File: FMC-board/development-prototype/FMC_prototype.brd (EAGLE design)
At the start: 103.8 x 69.8 mm, 65 parts, among them J1 DC_POWER_JACK-PJ-102AH, J2 DC_POWER_JACK-PJ-102AH

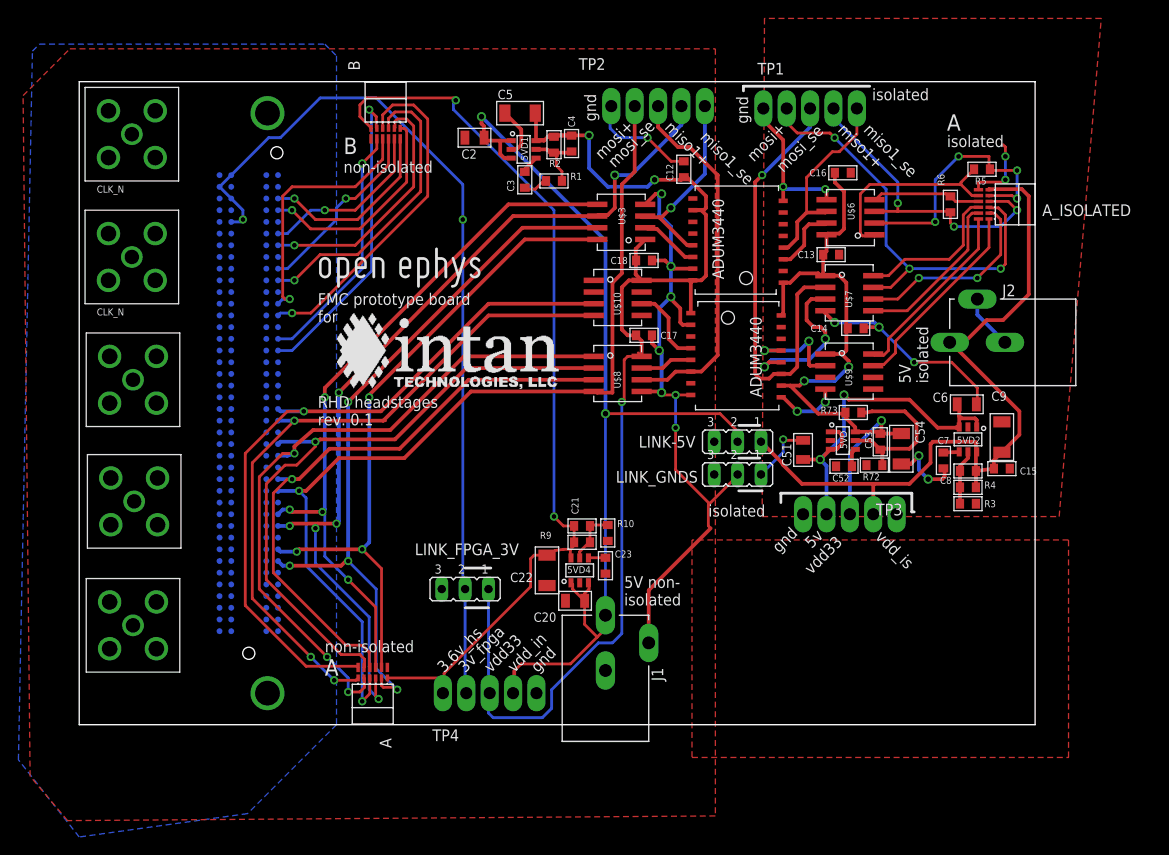
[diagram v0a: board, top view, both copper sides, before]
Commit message: small cleanups
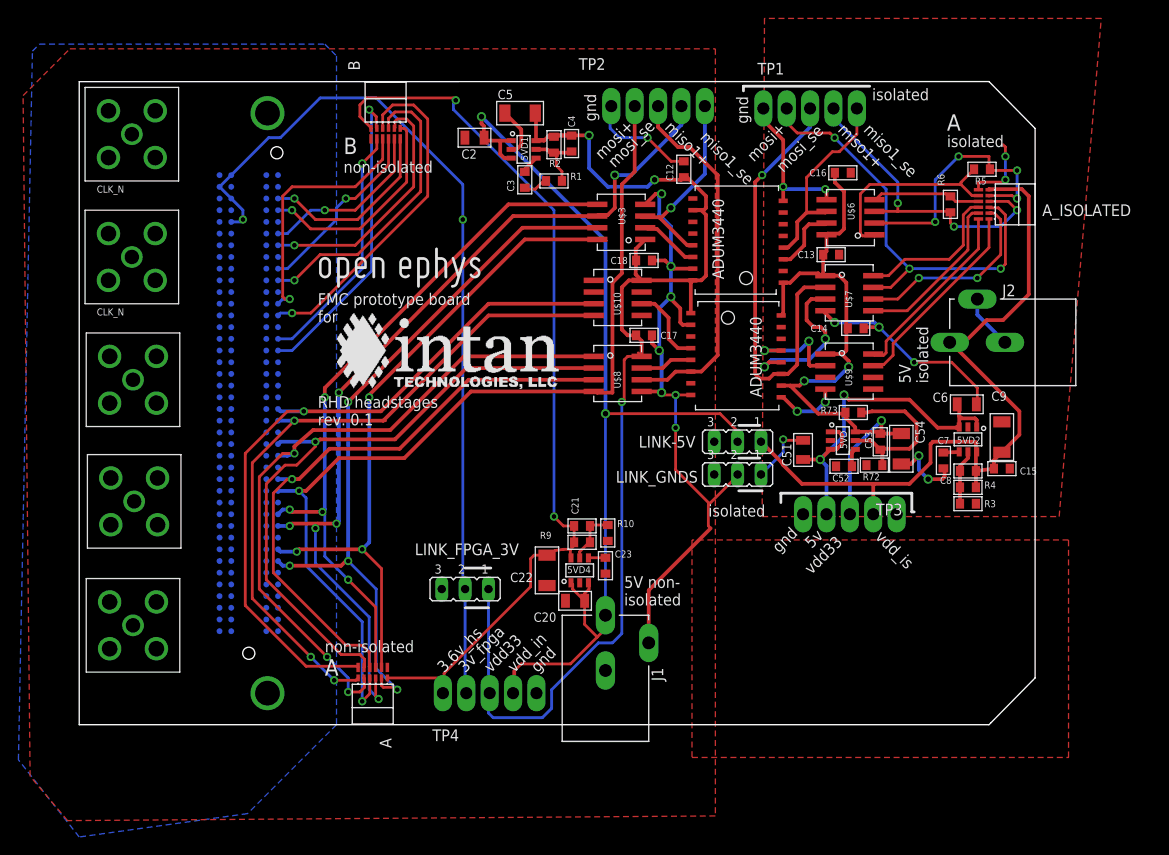
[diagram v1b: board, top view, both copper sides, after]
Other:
- outline, holes or cut-outs redrawn
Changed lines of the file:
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@@
 <setting verticaltext="up"/>
 </settings>
-<grid distance="0.01" unitdist="inch" unit="inch" style="dots" multiple="1" display="yes" altdistance="0.0125" altunitdist="inch" altunit="inch"/>
+<grid distance="0.01" unitdist="inch" unit="inch" style="lines" multiple="1" display="yes" altdistance="0.0125" altunitdist="inch" altunit="inch"/>
 <layers>
 <layer number="1" name="Top" color="42" fill="1" visible="yes" active="yes"/>
@@
 <board>
 <plain>
-<wire x1="0" y1="0" x2="103.81" y2="0" width="0" layer="20"/>
-<wire x1="103.81" y1="0" x2="103.81" y2="69.84" width="0" layer="20"/>
-<wire x1="103.81" y1="69.84" x2="0" y2="69.84" width="0" layer="20"/>
+<wire x1="0" y1="0" x2="98.806" y2="0" width="0" layer="20"/>
+<wire x1="98.806" y1="0" x2="98.984" y2="0.178" width="0" layer="20"/>
+<wire x1="98.984" y1="0.178" x2="103.81" y2="5.08" width="0" layer="20"/>
+<wire x1="103.81" y1="5.08" x2="103.81" y2="64.76" width="0" layer="20"/>
+<wire x1="103.81" y1="64.76" x2="98.816" y2="69.84" width="0" layer="20"/>
+<wire x1="98.816" y1="69.84" x2="98.806" y2="69.85" width="0" layer="20"/>
+<wire x1="98.806" y1="69.85" x2="0" y2="69.84" width="0" layer="20"/>
 <wire x1="0" y1="69.84" x2="0" y2="0" width="0" layer="20"/>
 <text x="1.905" y="57.785" size="0.762" layer="21">CLK_N</text>
@@
 <wire x1="57.658" y1="64.77" x2="57.658" y2="67.056" width="0.3048" layer="16"/>
 <wire x1="57.658" y1="67.056" x2="57.785" y2="67.183" width="0.3048" layer="16"/>
+<wire x1="21.59" y1="50.8" x2="21.59" y2="54.61" width="0" layer="19" extent="16-16"/>
+<wire x1="21.59" y1="46.99" x2="21.59" y2="50.8" width="0" layer="19" extent="16-16"/>
+<wire x1="21.59" y1="39.37" x2="21.59" y2="43.18" width="0" layer="19" extent="16-16"/>
 <wire x1="21.59" y1="27.94" x2="21.59" y2="31.75" width="0" layer="19" extent="16-16"/>
 <wire x1="21.59" y1="24.13" x2="21.59" y2="27.94" width="0" layer="19" extent="16-16"/>
+<wire x1="15.24" y1="54.61" x2="21.59" y2="54.61" width="0" layer="19" extent="16-16"/>
 </signal>
 <signal name="MISO2+">
@@
 <contactref element="A_ISOLATED" pad="T1"/>
 <wire x1="97.663" y1="54.9275" x2="97.663" y2="51.689" width="0.3048" layer="1"/>
-<wire x1="97.663" y1="51.689" x2="87.884" y2="41.91" width="0.3048" layer="1"/>
-<wire x1="87.884" y1="41.91" x2="87.884" y2="40.64" width="0.3048" layer="1"/>
-<wire x1="87.884" y1="40.64" x2="87.376" y2="40.132" width="0.3048" layer="1"/>
+<wire x1="97.663" y1="51.689" x2="87.63" y2="41.656" width="0.3048" layer="1"/>
+<wire x1="87.63" y1="41.656" x2="87.63" y2="40.386" width="0.3048" layer="1"/>
+<wire x1="87.63" y1="40.386" x2="87.376" y2="40.132" width="0.3048" layer="1"/>
 <wire x1="87.376" y1="40.132" x2="86.353" y2="40.132" width="0.3048" layer="1"/>
 <wire x1="86.353" y1="40.132" x2="86.226" y2="40.259" width="0.3048" layer="1"/>
@@
 <wire x1="81.026" y1="47.498" x2="78.74" y2="47.498" width="0.4064" layer="1"/>
 <wire x1="78.74" y1="47.498" x2="77.978" y2="46.736" width="0.4064" layer="1"/>
-<wire x1="77.978" y1="46.736" x2="77.978" y2="38.862" width="0.4064" layer="1"/>
-<wire x1="77.978" y1="38.862" x2="77.216" y2="38.1" width="0.4064" layer="1"/>
-<wire x1="77.216" y1="38.1" x2="76.235" y2="38.1" width="0.4064" layer="1"/>
+<wire x1="77.978" y1="46.736" x2="77.978" y2="39.116" width="0.4064" layer="1"/>
+<wire x1="77.978" y1="39.116" x2="76.962" y2="38.1" width="0.4064" layer="1"/>
+<wire x1="76.962" y1="38.1" x2="76.235" y2="38.1" width="0.4064" layer="1"/>
 <wire x1="79.375" y1="66.929" x2="79.375" y2="64.897" width="0.4064" layer="16"/>
 <wire x1="79.375" y1="64.897" x2="74.168" y2="59.69" width="0.4064" layer="16"/>
@@
 <contactref element="U$9" pad="P7"/>
 <wire x1="98.806" y1="54.9275" x2="98.806" y2="51.816" width="0.3048" layer="1"/>
-<wire x1="98.806" y1="51.816" x2="88.646" y2="41.656" width="0.3048" layer="1"/>
-<wire x1="88.646" y1="41.656" x2="88.646" y2="40.386" width="0.3048" layer="1"/>
-<wire x1="88.646" y1="40.386" x2="87.376" y2="39.116" width="0.3048" layer="1"/>
+<wire x1="98.806" y1="51.816" x2="88.392" y2="41.402" width="0.3048" layer="1"/>
+<wire x1="88.392" y1="41.402" x2="88.392" y2="40.132" width="0.3048" layer="1"/>
+<wire x1="88.392" y1="40.132" x2="87.376" y2="39.116" width="0.3048" layer="1"/>
 <wire x1="87.376" y1="39.116" x2="86.353" y2="39.116" width="0.3048" layer="1"/>
 <wire x1="86.353" y1="39.116" x2="86.226" y2="38.989" width="0.3048" layer="1"/>

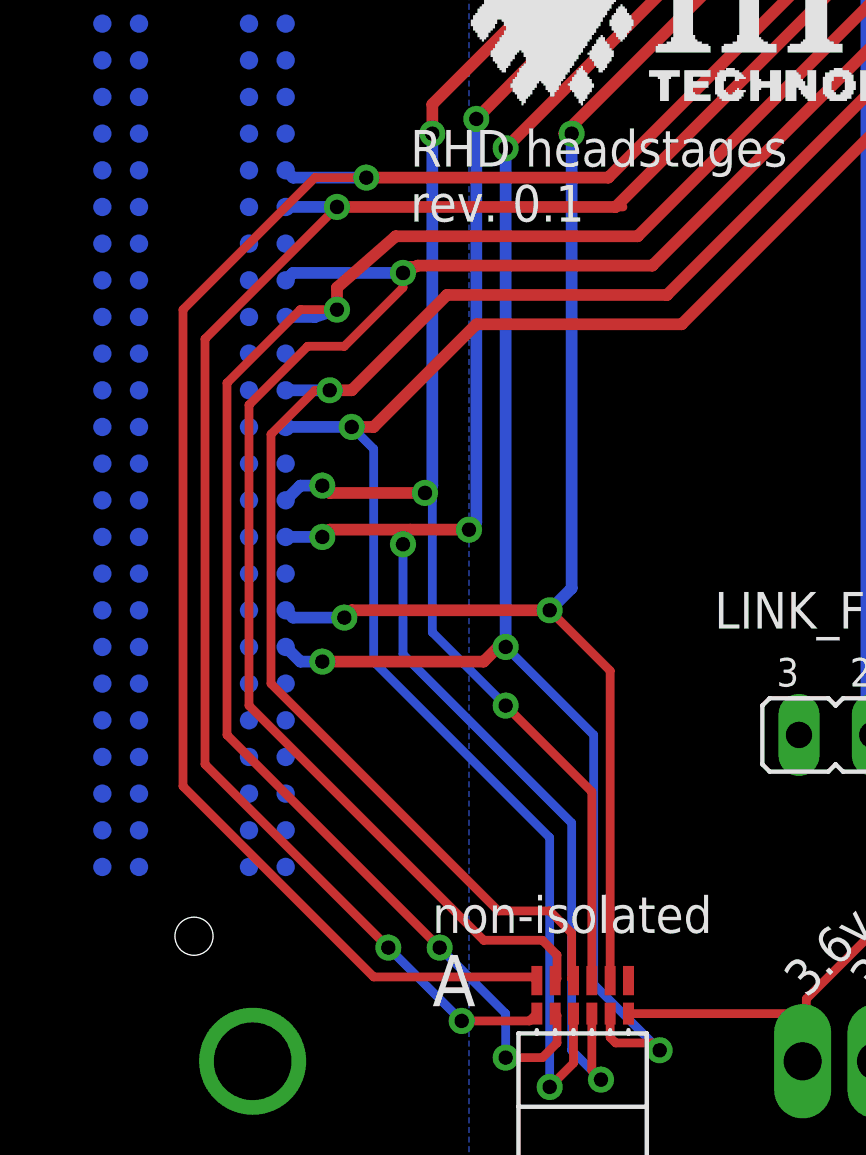
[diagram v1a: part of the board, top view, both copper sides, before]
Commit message: more small cleanups
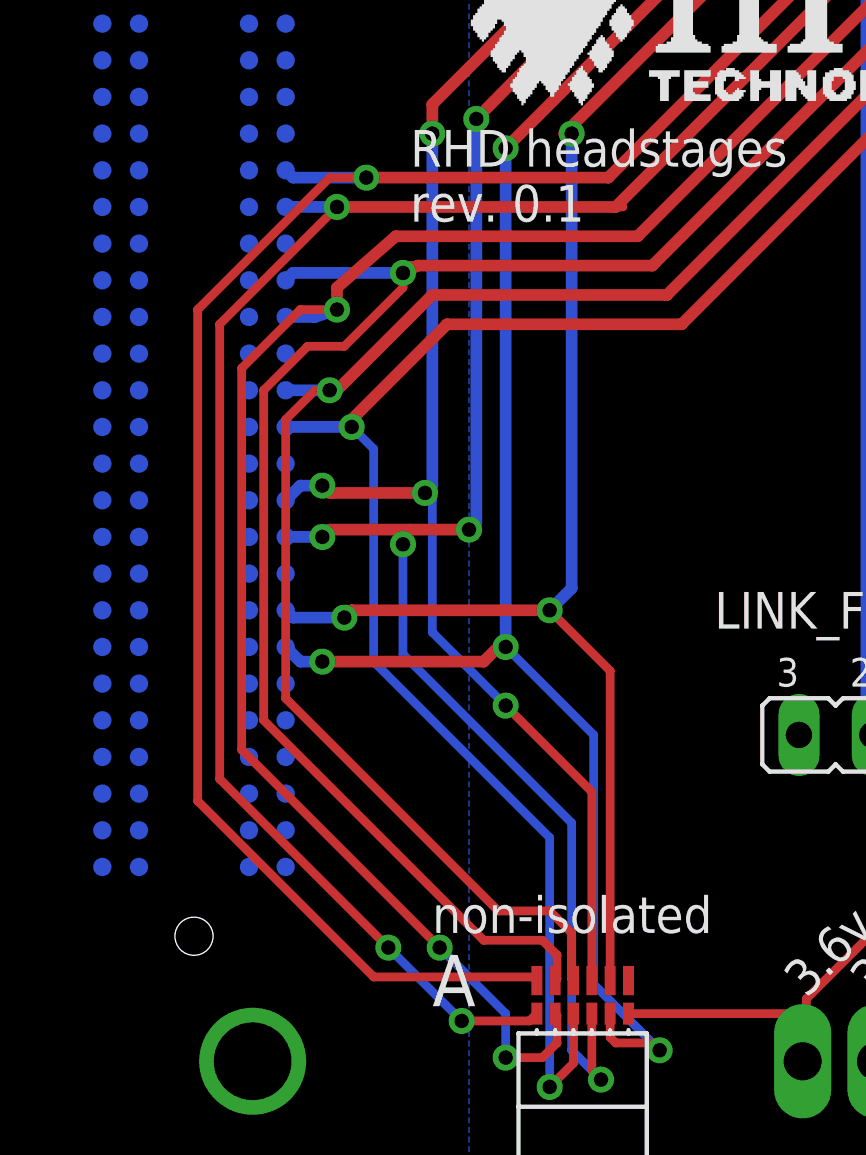
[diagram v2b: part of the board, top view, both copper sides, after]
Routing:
- net MOSI-: track 66.5 -> 65.6 mm
- net CS-: track 79.0 -> 78.3 mm
- net MOSI+: track 101.5 -> 102.0 mm
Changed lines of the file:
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@@
 <setting verticaltext="up"/>
 </settings>
-<grid distance="0.01" unitdist="inch" unit="inch" style="lines" multiple="1" display="yes" altdistance="0.0125" altunitdist="inch" altunit="inch"/>
+<grid distance="0.02" unitdist="inch" unit="inch" style="lines" multiple="1" display="yes" altdistance="0.0125" altunitdist="inch" altunit="inch"/>
 <layers>
 <layer number="1" name="Top" color="42" fill="1" visible="yes" active="yes"/>
-<layer number="16" name="Bottom" color="1" fill="1" visible="yes" active="yes"/>
+<layer number="16" name="Bottom" color="1" fill="1" visible="no" active="yes"/>
 <layer number="17" name="Pads" color="2" fill="1" visible="yes" active="yes"/>
 <layer number="18" name="Vias" color="2" fill="1" visible="yes" active="yes"/>
@@
 <wire x1="25.654" y1="30.226" x2="23.622" y2="28.194" width="0.3048" layer="1"/>
 <wire x1="23.622" y1="28.194" x2="22.352" y2="28.194" width="0.3048" layer="1"/>
-<wire x1="22.352" y1="28.194" x2="20.32" y2="26.162" width="0.3048" layer="1"/>
-<wire x1="20.32" y1="26.162" x2="20.32" y2="15.748" width="0.3048" layer="1"/>
-<wire x1="20.32" y1="15.748" x2="28.448" y2="7.62" width="0.3048" layer="1"/>
+<wire x1="22.352" y1="28.194" x2="20.828" y2="26.67" width="0.3048" layer="1"/>
+<wire x1="20.828" y1="26.67" x2="20.828" y2="15.24" width="0.3048" layer="1"/>
+<wire x1="20.828" y1="15.24" x2="28.448" y2="7.62" width="0.3048" layer="1"/>
 <wire x1="28.448" y1="7.62" x2="30.48" y2="7.62" width="0.3048" layer="1"/>
 <wire x1="30.48" y1="7.62" x2="30.988" y2="7.112" width="0.3048" layer="1"/>
@@
 <wire x1="22.606" y1="29.21" x2="21.59" y2="29.21" width="0.4064" layer="16"/>
 <wire x1="23.368" y1="29.464" x2="22.098" y2="29.464" width="0.3048" layer="1"/>
-<wire x1="22.098" y1="29.464" x2="19.558" y2="26.924" width="0.3048" layer="1"/>
-<wire x1="19.558" y1="26.924" x2="19.558" y2="14.732" width="0.3048" layer="1"/>
-<wire x1="19.558" y1="14.732" x2="26.924" y2="7.366" width="0.3048" layer="1"/>
+<wire x1="22.098" y1="29.464" x2="20.066" y2="27.432" width="0.3048" layer="1"/>
+<wire x1="20.066" y1="27.432" x2="20.066" y2="14.224" width="0.3048" layer="1"/>
+<wire x1="20.066" y1="14.224" x2="26.924" y2="7.366" width="0.3048" layer="1"/>
 <via x="26.924" y="7.366" extent="1-16" drill="0.5"/>
 <wire x1="26.924" y1="7.366" x2="29.21" y2="5.08" width="0.3048" layer="16"/>
@@
 <wire x1="55.88" y1="37.465" x2="42.291" y2="37.465" width="0.4064" layer="1"/>
 <wire x1="42.291" y1="37.465" x2="34.798" y2="29.972" width="0.4064" layer="1"/>
-<wire x1="34.798" y1="29.972" x2="27.178" y2="29.972" width="0.4064" layer="1"/>
-<wire x1="27.178" y1="29.972" x2="23.876" y2="26.67" width="0.4064" layer="1"/>
-<wire x1="23.876" y1="26.67" x2="23.114" y2="26.67" width="0.4064" layer="1"/>
+<wire x1="34.798" y1="29.972" x2="26.67" y2="29.972" width="0.4064" layer="1"/>
+<wire x1="26.67" y1="29.972" x2="23.368" y2="26.67" width="0.4064" layer="1"/>
+<wire x1="23.368" y1="26.67" x2="23.114" y2="26.67" width="0.4064" layer="1"/>
 <via x="23.114" y="26.67" extent="1-16" drill="0.5"/>
 <wire x1="23.114" y1="26.67" x2="21.59" y2="26.67" width="0.4064" layer="16"/>
-<wire x1="23.876" y1="26.67" x2="22.606" y2="26.67" width="0.3048" layer="1"/>
-<wire x1="22.606" y1="26.67" x2="21.082" y2="25.146" width="0.3048" layer="1"/>
-<wire x1="21.082" y1="25.146" x2="21.082" y2="16.51" width="0.3048" layer="1"/>
-<wire x1="21.082" y1="16.51" x2="28.956" y2="8.636" width="0.3048" layer="1"/>
+<wire x1="23.368" y1="26.67" x2="22.606" y2="26.67" width="0.3048" layer="1"/>
+<wire x1="22.606" y1="26.67" x2="21.59" y2="25.654" width="0.3048" layer="1"/>
+<wire x1="21.59" y1="25.654" x2="21.59" y2="16.002" width="0.3048" layer="1"/>
+<wire x1="21.59" y1="16.002" x2="28.956" y2="8.636" width="0.3048" layer="1"/>
 <wire x1="28.956" y1="8.636" x2="30.734" y2="8.636" width="0.3048" layer="1"/>
 <wire x1="30.734" y1="8.636" x2="31.496" y2="7.874" width="0.3048" layer="1"/>
@@
 <wire x1="55.88" y1="36.195" x2="42.545" y2="36.195" width="0.4064" layer="1"/>
 <wire x1="42.545" y1="36.195" x2="35.306" y2="28.956" width="0.4064" layer="1"/>
-<wire x1="35.306" y1="28.956" x2="28.194" y2="28.956" width="0.4064" layer="1"/>
-<wire x1="28.194" y1="28.956" x2="24.638" y2="25.4" width="0.4064" layer="1"/>
-<wire x1="24.638" y1="25.4" x2="23.876" y2="25.4" width="0.4064" layer="1"/>
+<wire x1="35.306" y1="28.956" x2="27.178" y2="28.956" width="0.4064" layer="1"/>
+<wire x1="27.178" y1="28.956" x2="23.622" y2="25.4" width="0.4064" layer="1"/>
+<wire x1="23.622" y1="25.4" x2="23.876" y2="25.4" width="0.4064" layer="1"/>
 <via x="23.876" y="25.4" extent="1-16" drill="0.5"/>
 <wire x1="23.876" y1="25.4" x2="21.59" y2="25.4" width="0.4064" layer="16"/>
@@
 <wire x1="24.384" y1="34.036" x2="21.844" y2="34.036" width="0.4064" layer="16"/>
 <wire x1="21.844" y1="34.036" x2="21.59" y2="34.29" width="0.4064" layer="16"/>
-<wire x1="24.384" y1="34.036" x2="22.606" y2="34.036" width="0.3048" layer="1"/>
-<wire x1="22.606" y1="34.036" x2="18.034" y2="29.464" width="0.3048" layer="1"/>
-<wire x1="18.034" y1="29.464" x2="18.034" y2="12.954" width="0.3048" layer="1"/>
-<wire x1="18.034" y1="12.954" x2="24.638" y2="6.35" width="0.3048" layer="1"/>
+<wire x1="24.384" y1="34.036" x2="23.114" y2="34.036" width="0.3048" layer="1"/>
+<wire x1="23.114" y1="34.036" x2="18.542" y2="29.464" width="0.3048" layer="1"/>
+<wire x1="18.542" y1="29.464" x2="18.542" y2="12.446" width="0.3048" layer="1"/>
+<wire x1="18.542" y1="12.446" x2="24.638" y2="6.35" width="0.3048" layer="1"/>
 <wire x1="24.638" y1="6.35" x2="30.1625" y2="6.35" width="0.3048" layer="1"/>
 <wire x1="30.1625" y1="6.35" x2="30.2895" y2="6.223" width="0.3048" layer="1"/>
@@
 <wire x1="23.368" y1="33.02" x2="21.59" y2="33.02" width="0.4064" layer="16"/>
 <wire x1="33.02" y1="33.02" x2="33.274" y2="33.02" width="0.3048" layer="1"/>
-<wire x1="23.368" y1="33.02" x2="18.796" y2="28.448" width="0.3048" layer="1"/>
-<wire x1="18.796" y1="28.448" x2="18.796" y2="13.716" width="0.3048" layer="1"/>
-<wire x1="18.796" y1="13.716" x2="25.146" y2="7.366" width="0.3048" layer="1"/>
+<wire x1="23.368" y1="33.02" x2="19.304" y2="28.956" width="0.3048" layer="1"/>
+<wire x1="19.304" y1="28.956" x2="19.304" y2="13.208" width="0.3048" layer="1"/>
+<wire x1="19.304" y1="13.208" x2="25.146" y2="7.366" width="0.3048" layer="1"/>
 <via x="25.146" y="7.366" extent="1-16" drill="0.5"/>
 <wire x1="25.146" y1="7.366" x2="27.686" y2="4.826" width="0.3048" layer="16"/>
